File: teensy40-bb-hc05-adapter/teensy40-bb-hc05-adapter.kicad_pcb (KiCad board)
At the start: 2 copper layers, 18 x 71.6 mm, 18 parts, among them J1 Conn_01x06_0.1_Header, J2 Conn_01x06_0.1_Socket, J3 Conn_01x08, J4 Conn_01x08, U1 74LVC1G17, U2 74LVC1G14, U3 Teensy4.0_WithBottomAndEdge

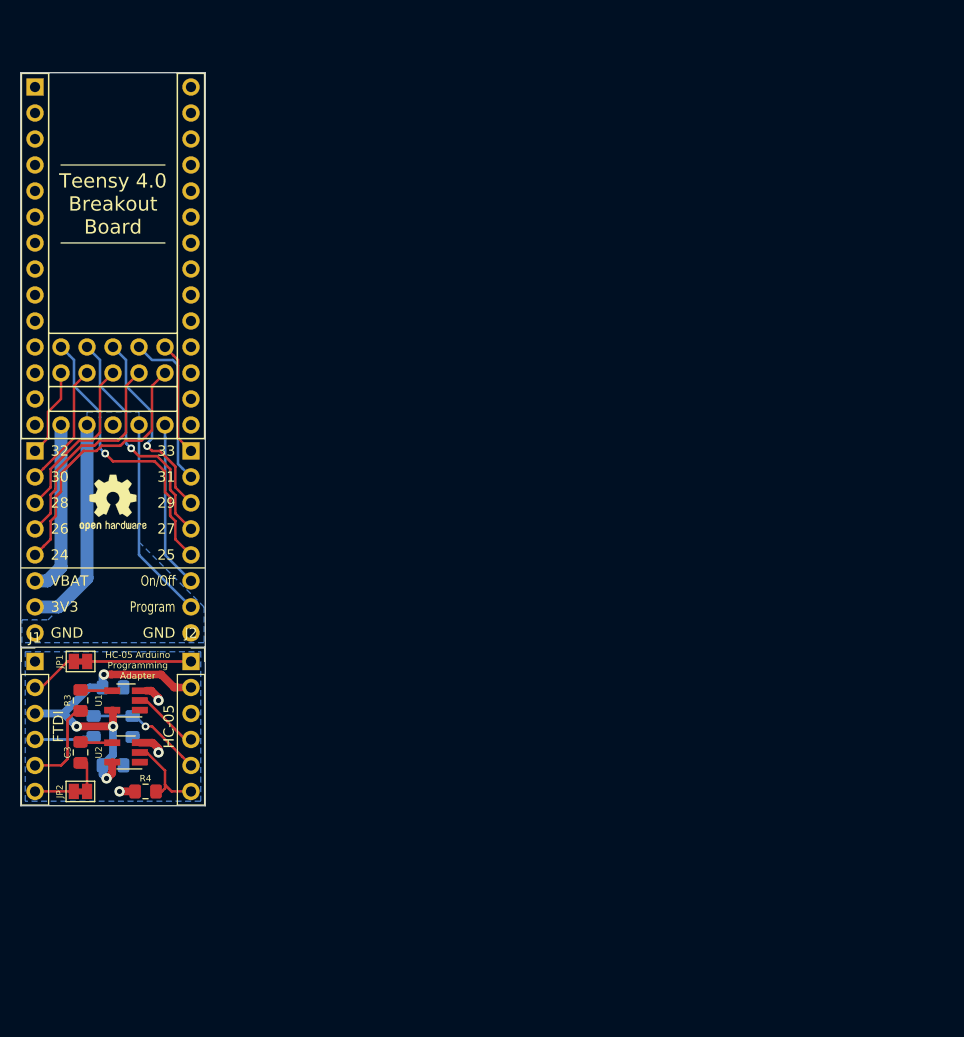
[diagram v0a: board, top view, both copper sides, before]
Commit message: Make panel
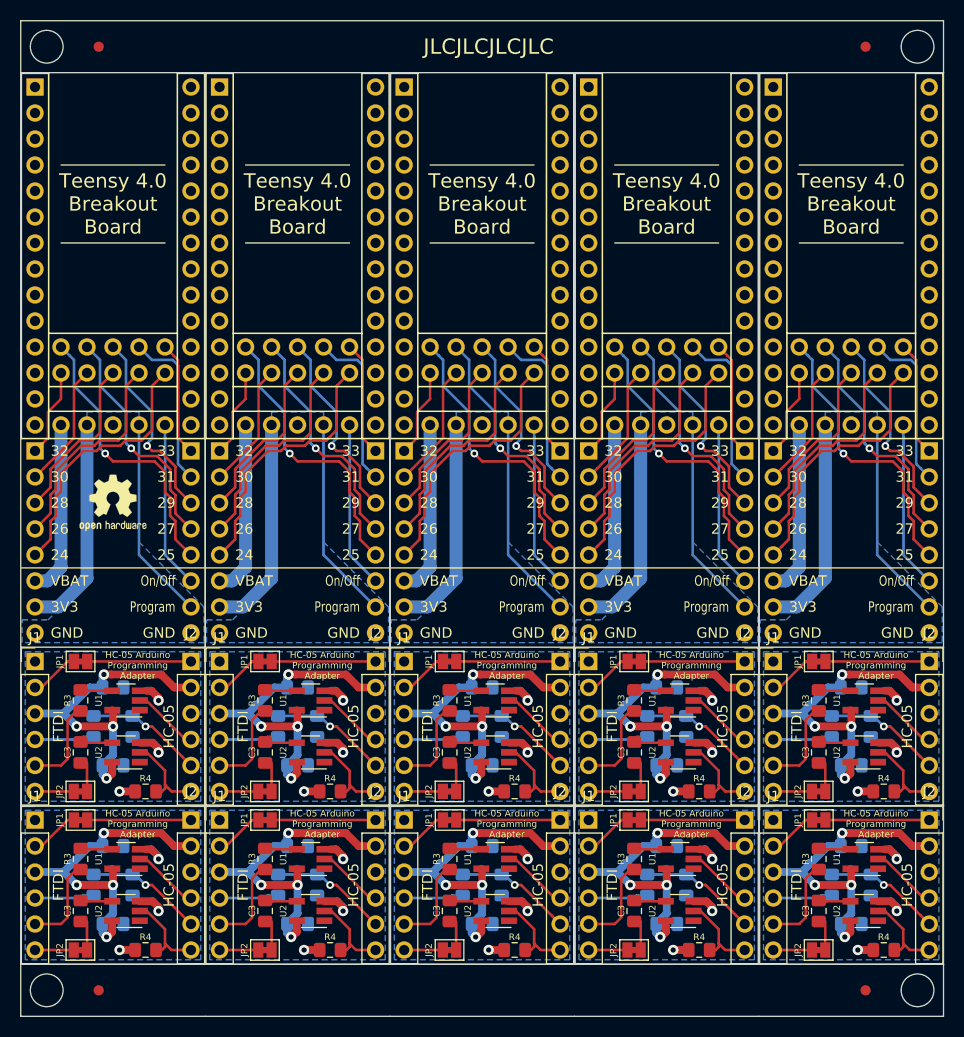
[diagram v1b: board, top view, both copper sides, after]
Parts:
- added C1: 0.1uF, Capacitor_SMD:C_0805_2012Metric_Pad1.15x1.40mm_HandSolder, B.Cu at (181.4, 125.0)
- added C1: 0.1uF, Capacitor_SMD:C_0805_2012Metric_Pad1.15x1.40mm_HandSolder, B.Cu at (163.3, 125.0)
- added C1: 0.1uF, Capacitor_SMD:C_0805_2012Metric_Pad1.15x1.40mm_HandSolder, B.Cu at (145.3, 125.0)
- added C1: 0.1uF, Capacitor_SMD:C_0805_2012Metric_Pad1.15x1.40mm_HandSolder, B.Cu at (127.3, 125.0)
- added C1: 0.1uF, Capacitor_SMD:C_0805_2012Metric_Pad1.15x1.40mm_HandSolder, B.Cu at (181.4, 109.5)
- added C1: 0.1uF, Capacitor_SMD:C_0805_2012Metric_Pad1.15x1.40mm_HandSolder, B.Cu at (163.3, 109.5)
- added C1: 0.1uF, Capacitor_SMD:C_0805_2012Metric_Pad1.15x1.40mm_HandSolder, B.Cu at (145.3, 109.5)
- added C1: 0.1uF, Capacitor_SMD:C_0805_2012Metric_Pad1.15x1.40mm_HandSolder, B.Cu at (127.3, 109.5)
- added C1: 0.1uF, Capacitor_SMD:C_0805_2012Metric_Pad1.15x1.40mm_HandSolder, B.Cu at (109.2, 125.0)
- added C2: 0.1uF, Capacitor_SMD:C_0805_2012Metric_Pad1.15x1.40mm_HandSolder, B.Cu at (181.4, 132.6)
- added C2: 0.1uF, Capacitor_SMD:C_0805_2012Metric_Pad1.15x1.40mm_HandSolder, B.Cu at (163.3, 132.6)
- added C2: 0.1uF, Capacitor_SMD:C_0805_2012Metric_Pad1.15x1.40mm_HandSolder, B.Cu at (145.3, 132.6)
- added C2: 0.1uF, Capacitor_SMD:C_0805_2012Metric_Pad1.15x1.40mm_HandSolder, B.Cu at (127.3, 132.6)
- added C2: 0.1uF, Capacitor_SMD:C_0805_2012Metric_Pad1.15x1.40mm_HandSolder, B.Cu at (181.4, 117.1)
- added C2: 0.1uF, Capacitor_SMD:C_0805_2012Metric_Pad1.15x1.40mm_HandSolder, B.Cu at (163.3, 117.1)
- added C2: 0.1uF, Capacitor_SMD:C_0805_2012Metric_Pad1.15x1.40mm_HandSolder, B.Cu at (145.3, 117.1)
- added C2: 0.1uF, Capacitor_SMD:C_0805_2012Metric_Pad1.15x1.40mm_HandSolder, B.Cu at (127.3, 117.1)
- added C2: 0.1uF, Capacitor_SMD:C_0805_2012Metric_Pad1.15x1.40mm_HandSolder, B.Cu at (109.2, 132.6)
- added C3: 0.1uF, Capacitor_SMD:C_0805_2012Metric_Pad1.15x1.40mm_HandSolder, F.Cu at (178.2, 131.3)
- added C3: 0.1uF, Capacitor_SMD:C_0805_2012Metric_Pad1.15x1.40mm_HandSolder, F.Cu at (160.2, 131.3)
- added C3: 0.1uF, Capacitor_SMD:C_0805_2012Metric_Pad1.15x1.40mm_HandSolder, F.Cu at (142.1, 131.3)
- added C3: 0.1uF, Capacitor_SMD:C_0805_2012Metric_Pad1.15x1.40mm_HandSolder, F.Cu at (124.1, 131.3)
- added C3: 0.1uF, Capacitor_SMD:C_0805_2012Metric_Pad1.15x1.40mm_HandSolder, F.Cu at (178.2, 115.8)
- added C3: 0.1uF, Capacitor_SMD:C_0805_2012Metric_Pad1.15x1.40mm_HandSolder, F.Cu at (160.2, 115.8)
- added C3: 0.1uF, Capacitor_SMD:C_0805_2012Metric_Pad1.15x1.40mm_HandSolder, F.Cu at (142.1, 115.8)
- added C3: 0.1uF, Capacitor_SMD:C_0805_2012Metric_Pad1.15x1.40mm_HandSolder, F.Cu at (124.1, 115.8)
- added C3: 0.1uF, Capacitor_SMD:C_0805_2012Metric_Pad1.15x1.40mm_HandSolder, F.Cu at (106.0, 131.3)
- added J1: Conn_01x06_0.1_Header, Connector_PinHeader_2.54mm:PinHeader_1x06_P2.54mm_Vertical, F.Cu at (173.7, 122.4)
- added J1: Conn_01x06_0.1_Header, Connector_PinHeader_2.54mm:PinHeader_1x06_P2.54mm_Vertical, F.Cu at (155.7, 122.4)
- added J1: Conn_01x06_0.1_Header, Connector_PinHeader_2.54mm:PinHeader_1x06_P2.54mm_Vertical, F.Cu at (137.7, 122.4)
- added J1: Conn_01x06_0.1_Header, Connector_PinHeader_2.54mm:PinHeader_1x06_P2.54mm_Vertical, F.Cu at (119.6, 122.4)
- added J1: Conn_01x06_0.1_Header, Connector_PinHeader_2.54mm:PinHeader_1x06_P2.54mm_Vertical, F.Cu at (173.7, 106.9)
- added J1: Conn_01x06_0.1_Header, Connector_PinHeader_2.54mm:PinHeader_1x06_P2.54mm_Vertical, F.Cu at (155.7, 106.9)
- added J1: Conn_01x06_0.1_Header, Connector_PinHeader_2.54mm:PinHeader_1x06_P2.54mm_Vertical, F.Cu at (137.7, 106.9)
- added J1: Conn_01x06_0.1_Header, Connector_PinHeader_2.54mm:PinHeader_1x06_P2.54mm_Vertical, F.Cu at (119.6, 106.9)
- added J1: Conn_01x06_0.1_Header, Connector_PinHeader_2.54mm:PinHeader_1x06_P2.54mm_Vertical, F.Cu at (101.6, 122.4)
- added J2: Conn_01x06_0.1_Socket, Connector_PinSocket_2.54mm:PinSocket_1x06_P2.54mm_Vertical, F.Cu at (189.0, 122.4)
- added J2: Conn_01x06_0.1_Socket, Connector_PinSocket_2.54mm:PinSocket_1x06_P2.54mm_Vertical, F.Cu at (170.9, 122.4)
- added J2: Conn_01x06_0.1_Socket, Connector_PinSocket_2.54mm:PinSocket_1x06_P2.54mm_Vertical, F.Cu at (152.9, 122.4)
- added J2: Conn_01x06_0.1_Socket, Connector_PinSocket_2.54mm:PinSocket_1x06_P2.54mm_Vertical, F.Cu at (134.9, 122.4)
- added J2: Conn_01x06_0.1_Socket, Connector_PinSocket_2.54mm:PinSocket_1x06_P2.54mm_Vertical, F.Cu at (189.0, 106.9)
- added J2: Conn_01x06_0.1_Socket, Connector_PinSocket_2.54mm:PinSocket_1x06_P2.54mm_Vertical, F.Cu at (170.9, 106.9)
- added J2: Conn_01x06_0.1_Socket, Connector_PinSocket_2.54mm:PinSocket_1x06_P2.54mm_Vertical, F.Cu at (152.9, 106.9)
- added J2: Conn_01x06_0.1_Socket, Connector_PinSocket_2.54mm:PinSocket_1x06_P2.54mm_Vertical, F.Cu at (134.9, 106.9)
- added J2: Conn_01x06_0.1_Socket, Connector_PinSocket_2.54mm:PinSocket_1x06_P2.54mm_Vertical, F.Cu at (116.8, 122.4)
- added J3: Conn_01x08, Connector_PinHeader_2.54mm:PinHeader_1x08_P2.54mm_Vertical, B.Cu at (173.7, 86.4)
- added J3: Conn_01x08, Connector_PinHeader_2.54mm:PinHeader_1x08_P2.54mm_Vertical, B.Cu at (155.7, 86.4)
- added J3: Conn_01x08, Connector_PinHeader_2.54mm:PinHeader_1x08_P2.54mm_Vertical, B.Cu at (137.7, 86.4)
- added J3: Conn_01x08, Connector_PinHeader_2.54mm:PinHeader_1x08_P2.54mm_Vertical, B.Cu at (119.6, 86.4)
- added J4: Conn_01x08, Connector_PinHeader_2.54mm:PinHeader_1x08_P2.54mm_Vertical, B.Cu at (189.0, 86.4)
- added J4: Conn_01x08, Connector_PinHeader_2.54mm:PinHeader_1x08_P2.54mm_Vertical, B.Cu at (170.9, 86.4)
- added J4: Conn_01x08, Connector_PinHeader_2.54mm:PinHeader_1x08_P2.54mm_Vertical, B.Cu at (152.9, 86.4)
- added J4: Conn_01x08, Connector_PinHeader_2.54mm:PinHeader_1x08_P2.54mm_Vertical, B.Cu at (134.9, 86.4)
- added JP1: SolderJumper_2_Bridged, Jumper:SolderJumper-2_P1.3mm_Bridged_Pad1.0x1.5mm, F.Cu at (178.2, 122.4)
- added JP1: SolderJumper_2_Bridged, Jumper:SolderJumper-2_P1.3mm_Bridged_Pad1.0x1.5mm, F.Cu at (160.2, 122.4)
- added JP1: SolderJumper_2_Bridged, Jumper:SolderJumper-2_P1.3mm_Bridged_Pad1.0x1.5mm, F.Cu at (142.1, 122.4)
- added JP1: SolderJumper_2_Bridged, Jumper:SolderJumper-2_P1.3mm_Bridged_Pad1.0x1.5mm, F.Cu at (124.1, 122.4)
- added JP1: SolderJumper_2_Bridged, Jumper:SolderJumper-2_P1.3mm_Bridged_Pad1.0x1.5mm, F.Cu at (178.2, 106.9)
- added JP1: SolderJumper_2_Bridged, Jumper:SolderJumper-2_P1.3mm_Bridged_Pad1.0x1.5mm, F.Cu at (160.2, 106.9)
- added JP1: SolderJumper_2_Bridged, Jumper:SolderJumper-2_P1.3mm_Bridged_Pad1.0x1.5mm, F.Cu at (142.1, 106.9)
- added JP1: SolderJumper_2_Bridged, Jumper:SolderJumper-2_P1.3mm_Bridged_Pad1.0x1.5mm, F.Cu at (124.1, 106.9)
- added JP1: SolderJumper_2_Bridged, Jumper:SolderJumper-2_P1.3mm_Bridged_Pad1.0x1.5mm, F.Cu at (106.0, 122.4)
- added JP2: SolderJumper_2_Bridged, Jumper:SolderJumper-2_P1.3mm_Bridged_Pad1.0x1.5mm, F.Cu at (178.2, 135.1)
- added JP2: SolderJumper_2_Bridged, Jumper:SolderJumper-2_P1.3mm_Bridged_Pad1.0x1.5mm, F.Cu at (160.1, 135.1)
- added JP2: SolderJumper_2_Bridged, Jumper:SolderJumper-2_P1.3mm_Bridged_Pad1.0x1.5mm, F.Cu at (142.1, 135.1)
- added JP2: SolderJumper_2_Bridged, Jumper:SolderJumper-2_P1.3mm_Bridged_Pad1.0x1.5mm, F.Cu at (124.1, 135.1)
- added JP2: SolderJumper_2_Bridged, Jumper:SolderJumper-2_P1.3mm_Bridged_Pad1.0x1.5mm, F.Cu at (178.2, 119.6)
- added JP2: SolderJumper_2_Bridged, Jumper:SolderJumper-2_P1.3mm_Bridged_Pad1.0x1.5mm, F.Cu at (160.1, 119.6)
- added JP2: SolderJumper_2_Bridged, Jumper:SolderJumper-2_P1.3mm_Bridged_Pad1.0x1.5mm, F.Cu at (142.1, 119.6)
- added JP2: SolderJumper_2_Bridged, Jumper:SolderJumper-2_P1.3mm_Bridged_Pad1.0x1.5mm, F.Cu at (124.1, 119.6)
- added JP2: SolderJumper_2_Bridged, Jumper:SolderJumper-2_P1.3mm_Bridged_Pad1.0x1.5mm, F.Cu at (106.0, 135.1)
- added R1: 1K, Resistor_SMD:R_0805_2012Metric_Pad1.15x1.40mm_HandSolder, B.Cu at (179.5, 128.8)
- added R1: 1K, Resistor_SMD:R_0805_2012Metric_Pad1.15x1.40mm_HandSolder, B.Cu at (161.4, 128.8)
- added R1: 1K, Resistor_SMD:R_0805_2012Metric_Pad1.15x1.40mm_HandSolder, B.Cu at (143.4, 128.8)
- added R1: 1K, Resistor_SMD:R_0805_2012Metric_Pad1.15x1.40mm_HandSolder, B.Cu at (125.4, 128.8)
- added R1: 1K, Resistor_SMD:R_0805_2012Metric_Pad1.15x1.40mm_HandSolder, B.Cu at (179.5, 113.3)
- added R1: 1K, Resistor_SMD:R_0805_2012Metric_Pad1.15x1.40mm_HandSolder, B.Cu at (161.4, 113.3)
- added R1: 1K, Resistor_SMD:R_0805_2012Metric_Pad1.15x1.40mm_HandSolder, B.Cu at (143.4, 113.3)
- added R1: 1K, Resistor_SMD:R_0805_2012Metric_Pad1.15x1.40mm_HandSolder, B.Cu at (125.4, 113.3)
- added R1: 1K, Resistor_SMD:R_0805_2012Metric_Pad1.15x1.40mm_HandSolder, B.Cu at (107.3, 128.8)
- added R2: 2K, Resistor_SMD:R_0805_2012Metric_Pad1.15x1.40mm_HandSolder, B.Cu at (183.3, 128.8)
- added R2: 2K, Resistor_SMD:R_0805_2012Metric_Pad1.15x1.40mm_HandSolder, B.Cu at (165.2, 128.8)
- added R2: 2K, Resistor_SMD:R_0805_2012Metric_Pad1.15x1.40mm_HandSolder, B.Cu at (147.2, 128.8)
- added R2: 2K, Resistor_SMD:R_0805_2012Metric_Pad1.15x1.40mm_HandSolder, B.Cu at (129.2, 128.8)
- added R2: 2K, Resistor_SMD:R_0805_2012Metric_Pad1.15x1.40mm_HandSolder, B.Cu at (183.3, 113.3)
- added R2: 2K, Resistor_SMD:R_0805_2012Metric_Pad1.15x1.40mm_HandSolder, B.Cu at (165.2, 113.3)
- added R2: 2K, Resistor_SMD:R_0805_2012Metric_Pad1.15x1.40mm_HandSolder, B.Cu at (147.2, 113.3)
- added R2: 2K, Resistor_SMD:R_0805_2012Metric_Pad1.15x1.40mm_HandSolder, B.Cu at (129.2, 113.3)
- added R2: 2K, Resistor_SMD:R_0805_2012Metric_Pad1.15x1.40mm_HandSolder, B.Cu at (111.1, 128.8)
- added R3: 100, Resistor_SMD:R_0805_2012Metric_Pad1.15x1.40mm_HandSolder, F.Cu at (178.2, 126.2)
- added R3: 100, Resistor_SMD:R_0805_2012Metric_Pad1.15x1.40mm_HandSolder, F.Cu at (160.2, 126.2)
- added R3: 100, Resistor_SMD:R_0805_2012Metric_Pad1.15x1.40mm_HandSolder, F.Cu at (142.1, 126.2)
- added R3: 100, Resistor_SMD:R_0805_2012Metric_Pad1.15x1.40mm_HandSolder, F.Cu at (124.1, 126.2)
- added R3: 100, Resistor_SMD:R_0805_2012Metric_Pad1.15x1.40mm_HandSolder, F.Cu at (178.2, 110.7)
- added R3: 100, Resistor_SMD:R_0805_2012Metric_Pad1.15x1.40mm_HandSolder, F.Cu at (160.2, 110.7)
- added R3: 100, Resistor_SMD:R_0805_2012Metric_Pad1.15x1.40mm_HandSolder, F.Cu at (142.1, 110.7)
- added R3: 100, Resistor_SMD:R_0805_2012Metric_Pad1.15x1.40mm_HandSolder, F.Cu at (124.1, 110.7)
- added R3: 100, Resistor_SMD:R_0805_2012Metric_Pad1.15x1.40mm_HandSolder, F.Cu at (106.0, 126.2)
- added R4: 10K, Resistor_SMD:R_0805_2012Metric_Pad1.15x1.40mm_HandSolder, F.Cu at (184.5, 135.1)
- added R4: 10K, Resistor_SMD:R_0805_2012Metric_Pad1.15x1.40mm_HandSolder, F.Cu at (166.5, 135.1)
- added R4: 10K, Resistor_SMD:R_0805_2012Metric_Pad1.15x1.40mm_HandSolder, F.Cu at (148.5, 135.1)
- added R4: 10K, Resistor_SMD:R_0805_2012Metric_Pad1.15x1.40mm_HandSolder, F.Cu at (130.4, 135.1)
- added R4: 10K, Resistor_SMD:R_0805_2012Metric_Pad1.15x1.40mm_HandSolder, F.Cu at (184.5, 119.6)
- added R4: 10K, Resistor_SMD:R_0805_2012Metric_Pad1.15x1.40mm_HandSolder, F.Cu at (166.5, 119.6)
- added R4: 10K, Resistor_SMD:R_0805_2012Metric_Pad1.15x1.40mm_HandSolder, F.Cu at (148.5, 119.6)
- added R4: 10K, Resistor_SMD:R_0805_2012Metric_Pad1.15x1.40mm_HandSolder, F.Cu at (130.4, 119.6)
- added R4: 10K, Resistor_SMD:R_0805_2012Metric_Pad1.15x1.40mm_HandSolder, F.Cu at (112.4, 135.1)
- added REF**: MountingHole_3.2mm_M3, MountingHole:MountingHole_3.2mm_M3, F.Cu at (187.8, 139.1)
- added REF**: MountingHole_3.2mm_M3, MountingHole:MountingHole_3.2mm_M3, F.Cu at (102.7, 139.1)
- added REF**: Fiducial_1mm_Mask3mm, Fiducial:Fiducial_1mm_Mask3mm, F.Cu at (107.8, 139.1)
- added REF**: Fiducial_1mm_Mask3mm, Fiducial:Fiducial_1mm_Mask3mm, F.Cu at (182.8, 139.1)
- added REF**: Fiducial_1mm_Mask3mm, Fiducial:Fiducial_1mm_Mask3mm, F.Cu at (182.8, 46.9)
- added REF**: MountingHole_3.2mm_M3, MountingHole:MountingHole_3.2mm_M3, F.Cu at (187.8, 46.9)
- added REF**: MountingHole_3.2mm_M3, MountingHole:MountingHole_3.2mm_M3, F.Cu at (102.7, 46.9)
- added REF**: Fiducial_1mm_Mask3mm, Fiducial:Fiducial_1mm_Mask3mm, F.Cu at (107.8, 46.9)
- added U1: 74LVC1G17, Package_TO_SOT_SMD:SOT-23-5_HandSoldering, F.Cu at (182.6, 126.2)
- added U1: 74LVC1G17, Package_TO_SOT_SMD:SOT-23-5_HandSoldering, F.Cu at (164.6, 126.2)
- added U1: 74LVC1G17, Package_TO_SOT_SMD:SOT-23-5_HandSoldering, F.Cu at (146.6, 126.2)
- added U1: 74LVC1G17, Package_TO_SOT_SMD:SOT-23-5_HandSoldering, F.Cu at (128.5, 126.2)
- added U1: 74LVC1G17, Package_TO_SOT_SMD:SOT-23-5_HandSoldering, F.Cu at (182.6, 110.7)
- added U1: 74LVC1G17, Package_TO_SOT_SMD:SOT-23-5_HandSoldering, F.Cu at (164.6, 110.7)
- added U1: 74LVC1G17, Package_TO_SOT_SMD:SOT-23-5_HandSoldering, F.Cu at (146.6, 110.7)
- added U1: 74LVC1G17, Package_TO_SOT_SMD:SOT-23-5_HandSoldering, F.Cu at (128.5, 110.7)
- added U1: 74LVC1G17, Package_TO_SOT_SMD:SOT-23-5_HandSoldering, F.Cu at (110.5, 126.2)
- added U2: 74LVC1G14, Package_TO_SOT_SMD:SOT-23-5_HandSoldering, F.Cu at (182.6, 131.3)
- added U2: 74LVC1G14, Package_TO_SOT_SMD:SOT-23-5_HandSoldering, F.Cu at (164.6, 131.3)
- added U2: 74LVC1G14, Package_TO_SOT_SMD:SOT-23-5_HandSoldering, F.Cu at (146.6, 131.3)
- added U2: 74LVC1G14, Package_TO_SOT_SMD:SOT-23-5_HandSoldering, F.Cu at (128.5, 131.3)
- added U2: 74LVC1G14, Package_TO_SOT_SMD:SOT-23-5_HandSoldering, F.Cu at (182.6, 115.8)
- added U2: 74LVC1G14, Package_TO_SOT_SMD:SOT-23-5_HandSoldering, F.Cu at (164.6, 115.8)
- added U2: 74LVC1G14, Package_TO_SOT_SMD:SOT-23-5_HandSoldering, F.Cu at (146.6, 115.8)
- added U2: 74LVC1G14, Package_TO_SOT_SMD:SOT-23-5_HandSoldering, F.Cu at (128.5, 115.8)
- added U2: 74LVC1G14, Package_TO_SOT_SMD:SOT-23-5_HandSoldering, F.Cu at (110.5, 131.3)
- added U3: Teensy4.0_WithBottomAndEdge, nibelung:Teensy40_Socket_WithBottomAndEdge, F.Cu at (181.4, 50.8)
- added U3: Teensy4.0_WithBottomAndEdge, nibelung:Teensy40_Socket_WithBottomAndEdge, F.Cu at (163.3, 50.8)
- added U3: Teensy4.0_WithBottomAndEdge, nibelung:Teensy40_Socket_WithBottomAndEdge, F.Cu at (145.3, 50.8)
- added U3: Teensy4.0_WithBottomAndEdge, nibelung:Teensy40_Socket_WithBottomAndEdge, F.Cu at (127.3, 50.8)
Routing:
- net +5V: track 49.7 -> 412.4 mm, vias 4 -> 40
- net Net-(J4-Pad5): track 28.0 -> 139.8 mm, vias 1 -> 5
- net /hc05-adapter/BT_RX: track 11.5 -> 115.3 mm, vias 1 -> 10
- net Net-(J3-Pad5): track 25.8 -> 128.8 mm
- net Net-(J4-Pad4): track 23.0 -> 115.1 mm, vias 1 -> 5
- net /hc05-adapter/BT_EN: track 10.1 -> 101.5 mm
- net /hc05-adapter/RX: track 9.52 -> 95.2 mm
- net Net-(J3-Pad4): track 21.3 -> 106.3 mm
- net +3V3: track 21.2 -> 106.1 mm
- net Net-(J4-Pad7): track 19.9 -> 99.4 mm
- net Net-(J4-Pad3): track 19.3 -> 96.3 mm, vias 1 -> 5
- net /hc05-adapter/BT_RST: track 8.10 -> 81.0 mm
- net Net-(J3-Pad3): track 16.6 -> 83.0 mm
- net Net-(J4-Pad6): track 16.3 -> 81.5 mm
- net Net-(J4-Pad2): track 16.0 -> 80.0 mm
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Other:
- board size 18 x 71.6 mm -> 90.2 x 97.3 mm
- board text added: "Grid for edges: 2.5 mil"
- board text added: "JLCJLCJLCJLC"
